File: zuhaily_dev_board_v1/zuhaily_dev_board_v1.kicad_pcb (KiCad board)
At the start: 2 copper layers, 53 parts, among them J1 USB_B_Micro, J2 SD_Card, J3 DC_JACK, Q1 FS8205A, SW1 SW_DPDT_x2, SW2 SW_SPST, U1 74LVC245, U10 DW-01, U2 LM1117-5.0, U3 CH340G, U4 LM1117-3.3, U5 ATmega328-PU, U6 ESP-01v090, U7 TP4056, U8 LMV358, Y1 Crystal_12MHz, Y2 Crystal_16MHz

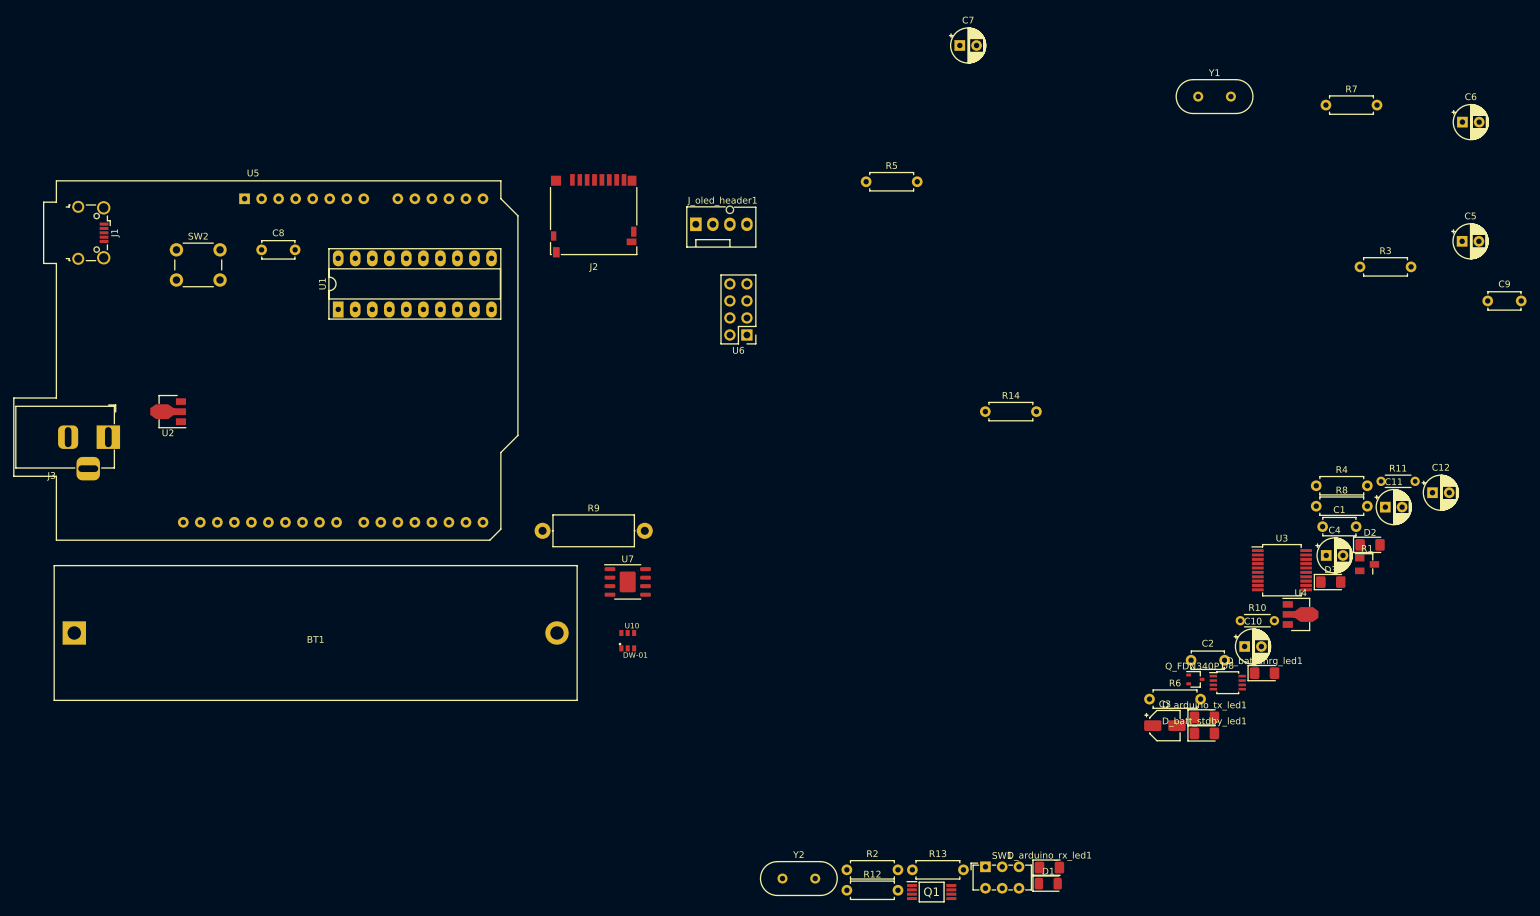
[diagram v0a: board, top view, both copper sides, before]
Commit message: generated pcb
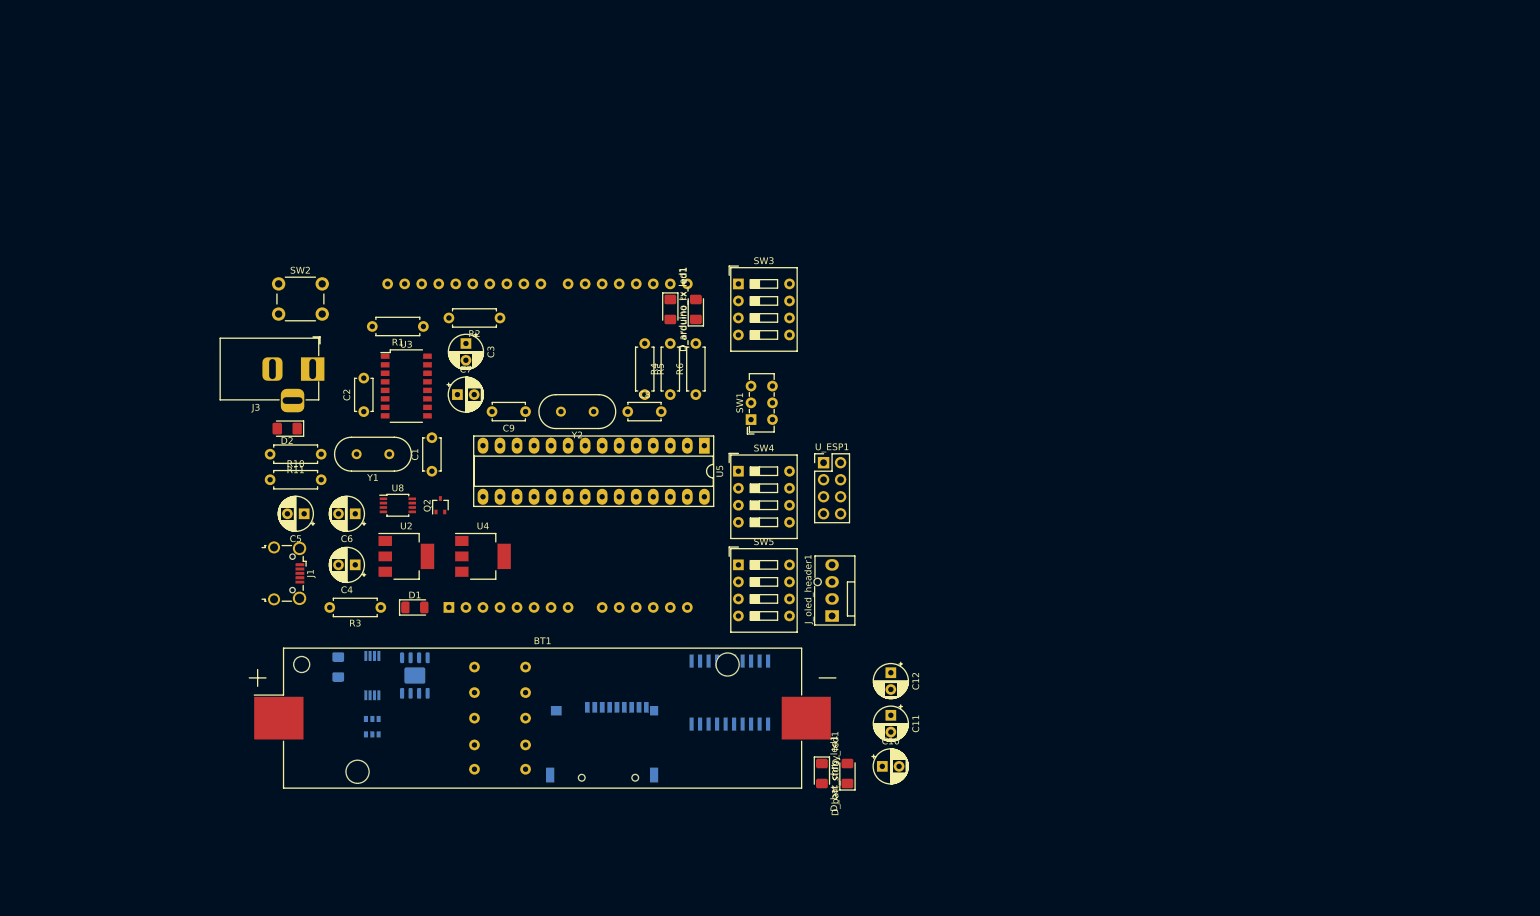
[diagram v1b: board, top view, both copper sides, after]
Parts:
- removed Q_FDN340P1: MOSFET_P_CH, Package_TO_SOT_SMD:SOT-323_SC-70
- removed R9: 0.4, Resistor_THT:R_Axial_DIN0414_L11.9mm_D4.5mm_P15.24mm_Horizontal
- removed U6: ESP-01v090, Connector_PinHeader_2.54mm:PinHeader_2x04_P2.54mm_Vertical
- added J4: Conn_01x32_Female, Module:Arduino_UNO_R3, B.Cu at (82.5, 109.2)
- added Q2: FDN340P, Package_TO_SOT_SMD:SOT-323_SC-70, F.Cu at (81.3, 94.0)
- added SW3: SW_DIP_x04, Button_Switch_THT:SW_DIP_SPSTx04_Slide_9.78x12.34mm_W7.62mm_P2.54mm, F.Cu at (125.7, 61.0)
- added SW4: SW_DIP_x04, Button_Switch_THT:SW_DIP_SPSTx04_Slide_9.78x12.34mm_W7.62mm_P2.54mm, F.Cu at (125.7, 88.9)
- added SW5: SW_DIP_x04, Button_Switch_THT:SW_DIP_SPSTx04_Slide_9.78x12.34mm_W7.62mm_P2.54mm, F.Cu at (125.7, 102.9)
- added U_ESP1: ESP-01v090, Connector_PinHeader_2.54mm:PinHeader_2x04_P2.54mm_Vertical, F.Cu at (138.4, 87.6)
- BT1: footprint Battery:BatteryHolder_MPD_BH-18650-PC2 -> Battery:BatteryHolder_Keystone_1042_1x18650
- C10: value 0.1u -> 0.1uF
- C3: footprint Capacitor_SMD:CP_Elec_4x3.9 -> Capacitor_THT:CP_Radial_D5.0mm_P2.50mm
- C7: value C -> 0.1uF
- D2: value DIODE -> D
- D3, Q1, R12, R13, R14, R7, R8, U10, U7: moved to B.Cu
- J2: value SD_Card -> Micro_SD_Card; footprint Connector_Card:microSD_HC_Hirose_DM3D-SF -> sd_card_pretty:Conn_uSDcard; moved to B.Cu
- R1: footprint Package_TO_SOT_SMD:SuperSOT-3 -> Resistor_THT:R_Axial_DIN0207_L6.3mm_D2.5mm_P7.62mm_Horizontal
- R10, R11: footprint Resistor_THT:R_Axial_DIN0204_L3.6mm_D1.6mm_P5.08mm_Horizontal -> Resistor_THT:R_Axial_DIN0207_L6.3mm_D2.5mm_P7.62mm_Horizontal
- U1: footprint Package_DIP:DIP-20_W7.62mm_Socket_LongPads -> Package_SO:SOIC-20W_7.5x12.8mm_P1.27mm; moved to B.Cu
- U2, U4: footprint Package_TO_SOT_SMD:SOT-89-3 -> Package_TO_SOT_SMD:SOT-223
- U3: footprint Package_SO:SSOP-20_5.3x7.2mm_P0.65mm -> Package_SO:SOP-16_4.4x10.4mm_P1.27mm
- U5: footprint Module:Arduino_UNO_R3 -> Package_DIP:DIP-28_W7.62mm_Socket_LongPads
- moved C5 177.4 mm to (61.0, 95.2), turned to 180 degrees
- moved C6 175.2 mm to (68.6, 95.2), turned to 180 degrees
- moved D2 162.4 mm to (58.4, 82.5), turned to 180 degrees
- moved R11 158.1 mm to (63.5, 86.4), turned to 180 degrees
- moved R3 154.6 mm to (72.4, 109.2), turned to 180 degrees
- moved R7 150.4 mm to (94.0, 125.7), turned to 180 degrees
- moved D3 148.6 mm to (66.0, 118.1), turned to 270 degrees
- moved R10 146.2 mm to (55.9, 90.2)
- moved R1 145.2 mm to (78.7, 67.3), turned to 180 degrees
- moved C4 144.8 mm to (68.6, 102.9), turned to 180 degrees
- moved C9 144.5 mm to (94.0, 80.0), turned to 180 degrees
- moved U3 133.5 mm to (76.2, 76.2)
- moved C1 133.1 mm to (80.0, 88.9), turned to 90 degrees
- moved Y1 131.9 mm to (73.7, 86.4), turned to 180 degrees
- moved C2 128.8 mm to (69.8, 80.0), turned to 90 degrees
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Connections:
- C3 pad 1: /5V_REGULATED -> /5V_FILTERED
- C4 pad 1: /5V_REGULATED -> /5V_FILTERED
- C5 pad 1: /5V_REGULATED -> /5V_FILTERED
- C6 pad 1: /5V_REGULATED -> /5V_FILTERED
- D1 pad 2: /5V_REGULATED -> /5V_FILTERED
- D2 pad 1: Net-(D2-Pad1) -> /5V_REGULATOR_IN
- D2 pad 2: /5V_REGULATOR_IN -> Net-(D2-Pad2)
- D3 pad 1: (no net) -> /5V_FILTERED
- D3 pad 2: (no net) -> /BATT_OUT_POSITIVE
- J2 pad 1: /LEVEL_SHIFT_SD_CS -> Net-(J2-Pad1)
- J2 pad 2: /LEVEL_SHIFT_SD_MOSI -> /LEVEL_SHIFT_SD_CS
- J2 pad 3: GND -> /LEVEL_SHIFT_SD_MOSI
- J2 pad 7: /ARDUINO_SD_MISO -> Net-(J2-Pad7)
- J2 pad 9: Net-(J2-Pad9) -> GND
- J3 pad 2: Net-(D2-Pad1) -> Net-(D2-Pad2)
- R4 pad 1: /5V_REGULATED -> /5V_FILTERED
- R5 pad 2: /5V_REGULATED -> /5V_FILTERED
- R6 pad 1: /5V_REGULATED -> /5V_FILTERED
- U1 pad 5: /ARDUINO_LEVEL_SHIFT_SCK -> Net-(SW3-Pad8)
- U1 pad 6: /ARDUINO_LEVEL_SHIFT_CS -> Net-(SW3-Pad7)
- U1 pad 7: /ARDUINO_LEVEL_SHIFT_MOSI -> Net-(SW3-Pad6)
- U2 pad 2: /5V_REGULATED -> /5V_FILTERED
- U3 pad 16: /5V_REGULATED -> /5V_FILTERED
- U4 pad 3: /5V_REGULATED -> /5V_FILTERED
- U5 pad 11: Net-(U5-Pad11) -> /PD_5
- U5 pad 12: Net-(U5-Pad12) -> /PD_6
- U5 pad 13: Net-(U5-Pad13) -> /PD_7
- U5 pad 14: Net-(U5-Pad14) -> /PB_0
- U5 pad 15: Net-(U5-Pad15) -> /PB_1
- U5 pad 2: Net-(U5-Pad2) -> /ARDUINO_RX
- U5 pad 20: /5V_REGULATED -> /5V_FILTERED
- U5 pad 21: /5V_REGULATED -> /5V_FILTERED
- U5 pad 23: Net-(U5-Pad23) -> /PC_0
- U5 pad 24: Net-(U5-Pad24) -> /PC_1
- U5 pad 25: Net-(U5-Pad25) -> /PC_2
- U5 pad 26: Net-(U5-Pad26) -> /PC_3
- U5 pad 27: Net-(U5-Pad27) -> /PC_4
- U5 pad 28: Net-(U5-Pad28) -> /PC_5
- U5 pad 3: Net-(U5-Pad3) -> /ARDUINO_TX
- U5 pad 4: Net-(U5-Pad4) -> /PD_2
- U5 pad 5: Net-(U5-Pad5) -> /PD_3
- U5 pad 6: Net-(U5-Pad6) -> /PD_4
- U5 pad 7: /5V_REGULATED -> /5V_FILTERED
- U8 pad 4: Net-(U8-Pad4) -> GND
- U8 pad 8: Net-(U8-Pad8) -> /5V_FILTERED
